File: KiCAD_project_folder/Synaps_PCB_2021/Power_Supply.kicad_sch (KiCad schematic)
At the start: 23 parts, among them J1 USB_C_Receptacle, U4 1101M2S3CQE2, U5 1101M2S3CQE2

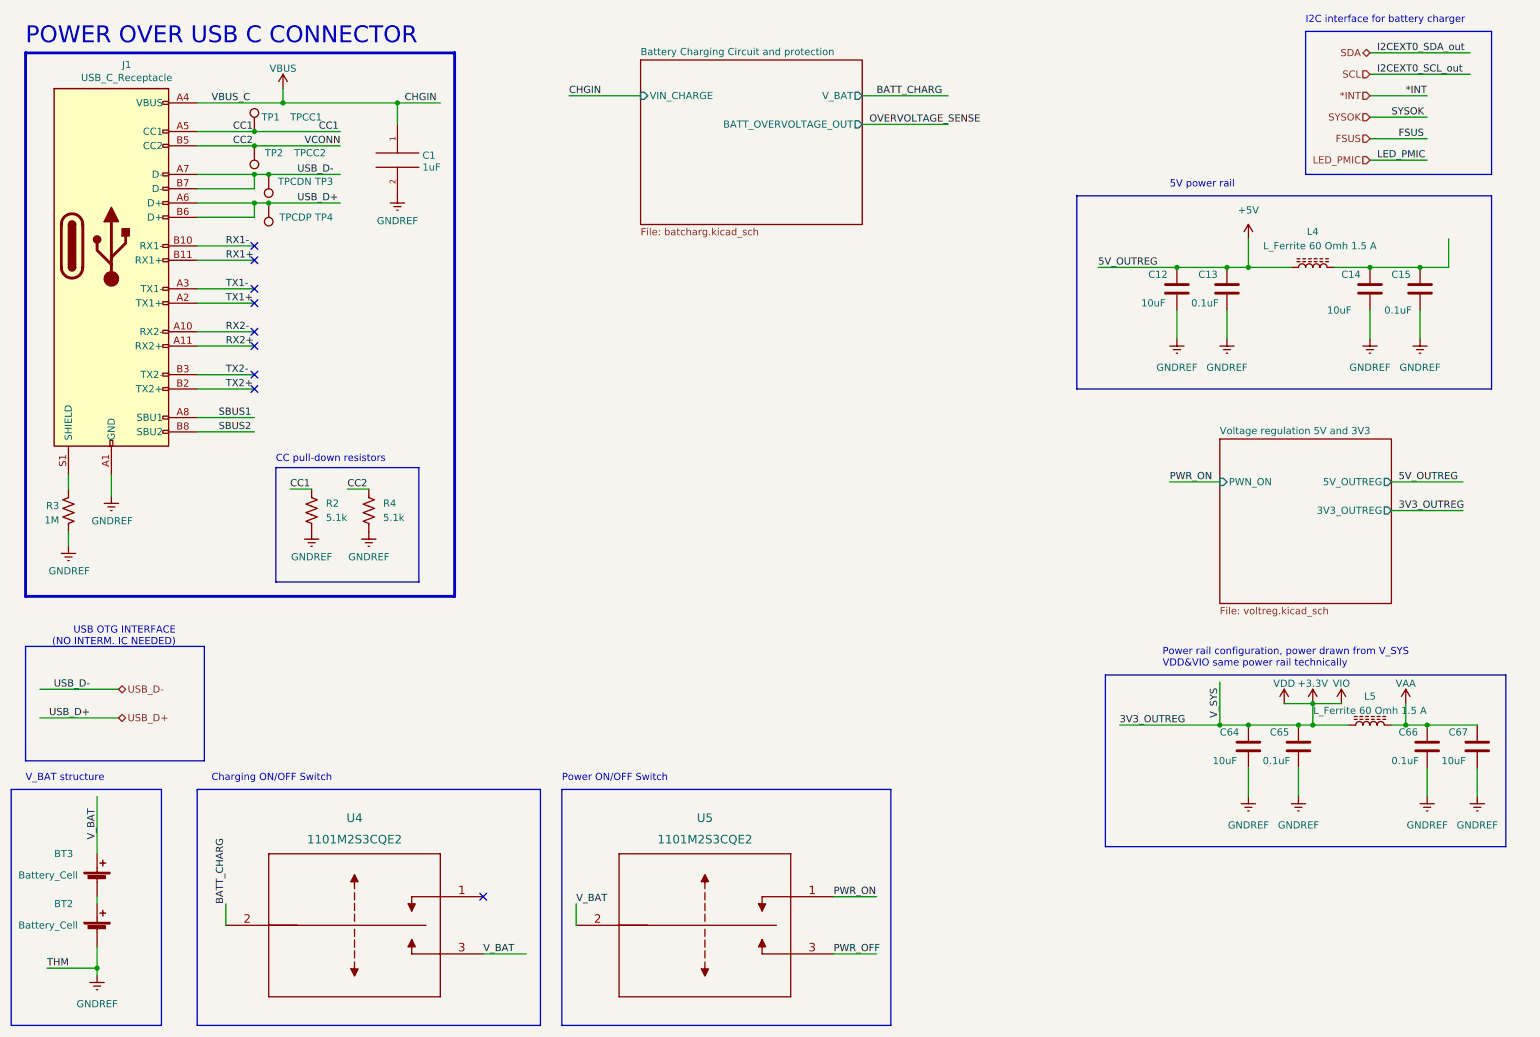
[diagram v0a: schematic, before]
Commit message: schematic finished
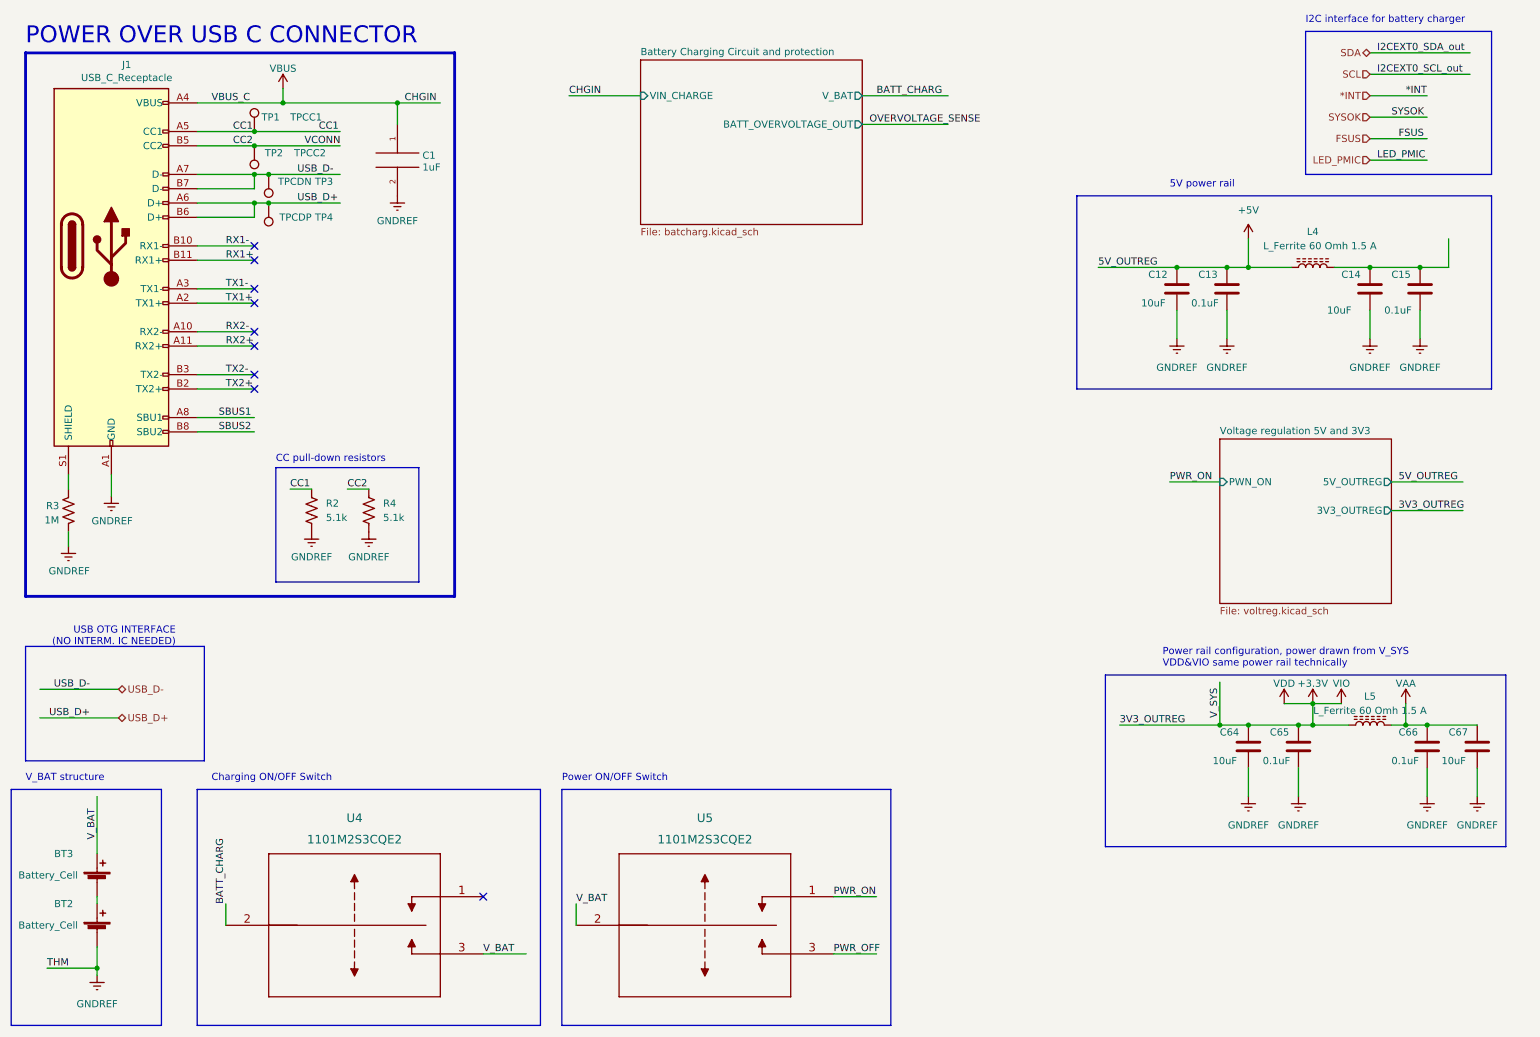
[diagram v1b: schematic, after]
